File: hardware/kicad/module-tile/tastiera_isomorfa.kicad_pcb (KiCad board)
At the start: 2 copper layers, 87 x 97.2 mm, 67 parts, among them J101 Conn_LEFT, J102 Conn_TOP, J103 Conn_BOTTOM, J104 Conn_RIGHT, J105 BTNs_L_MSB, J106 BTNs_L_LSB, J107 BTNs_MSB, J108 BTNs_LSB, SW101 SW_Push, SW102 SW_Push, SW103 SW_Push, SW104 SW_Push, SW105 SW_Push, SW106 SW_Push, SW107 SW_Push, SW108 SW_Push, SW109 SW_Push, SW110 SW_Push, SW111 SW_Push, SW112 SW_Push, U101 74AUC2G126, U102 74AUC2G08, U103 74HC165, U104 74HC165, U105 74AHC1G04, U106 74LVC2G32, U107 74AUC2G125, U108 74LVC2G74, U109 74LS161

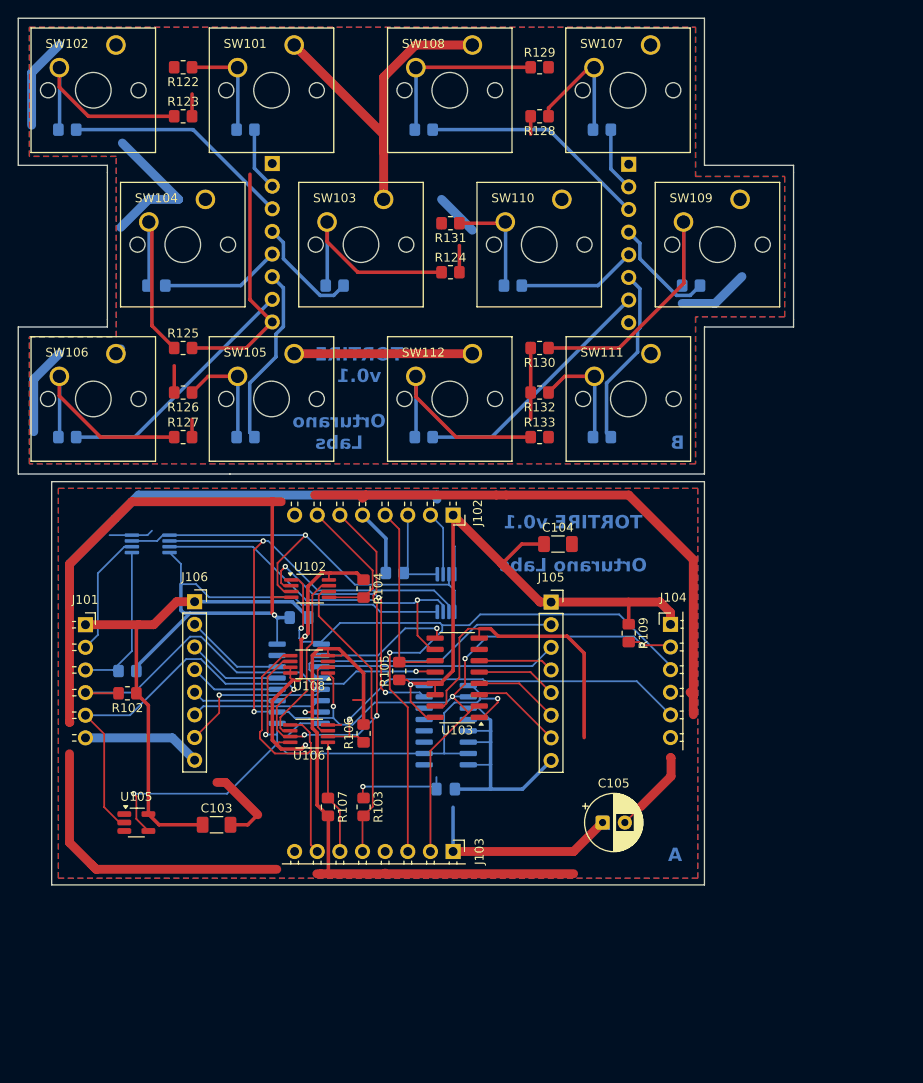
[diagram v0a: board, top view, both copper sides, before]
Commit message: Create gerber files
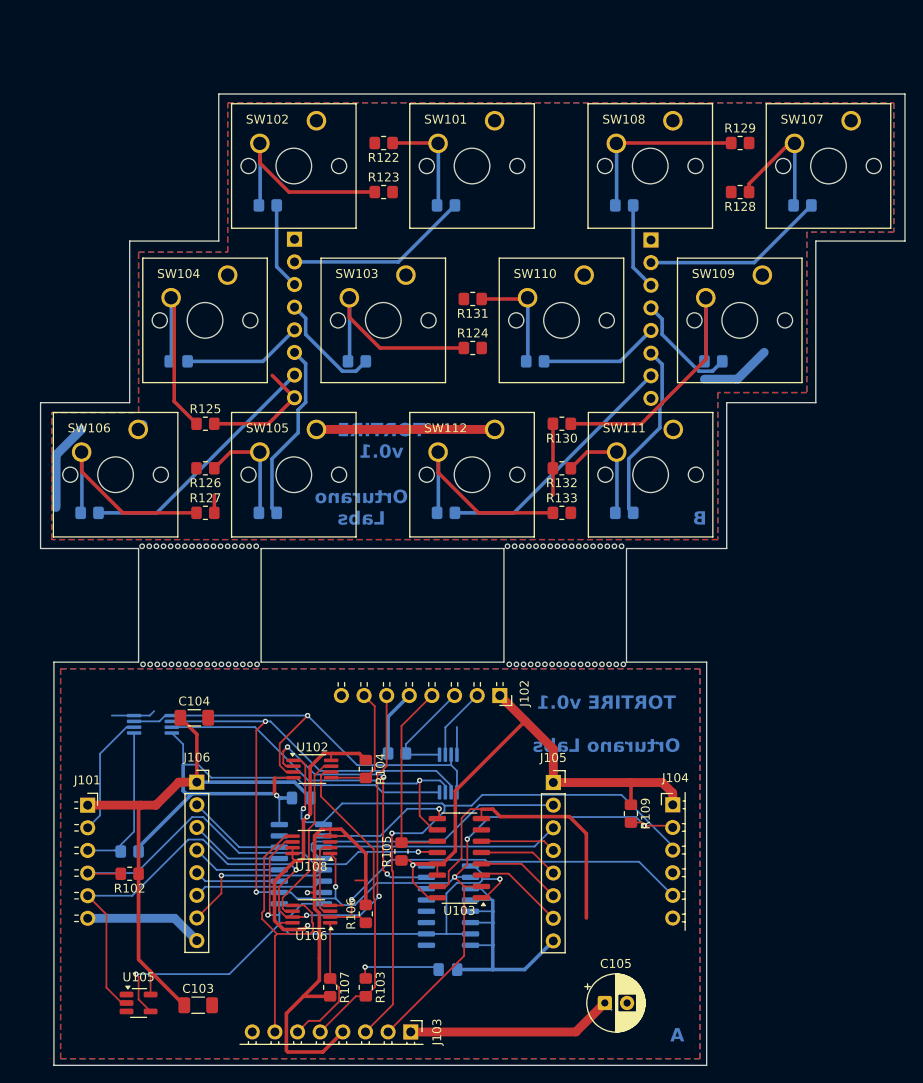
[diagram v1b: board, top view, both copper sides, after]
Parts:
- added REF**10: Senza-titolo, Senza-titolo, F.Cu at (124.5, 95.8)
- added REF**10: Senza-titolo, Senza-titolo, F.Cu at (166.5, 109.0)
- added REF**10: Senza-titolo, Senza-titolo, F.Cu at (124.6, 109.0)
- added REF**10: Senza-titolo, Senza-titolo, F.Cu at (165.5, 95.8)
- added REF**11: Senza-titolo, Senza-titolo, F.Cu at (125.3, 95.8)
- added REF**11: Senza-titolo, Senza-titolo, F.Cu at (166.3, 95.8)
- added REF**11: Senza-titolo, Senza-titolo, F.Cu at (167.3, 109.0)
- added REF**11: Senza-titolo, Senza-titolo, F.Cu at (125.4, 109.0)
- added REF**12: Senza-titolo, Senza-titolo, F.Cu at (126.1, 95.8)
- added REF**12: Senza-titolo, Senza-titolo, F.Cu at (126.2, 109.0)
- added REF**12: Senza-titolo, Senza-titolo, F.Cu at (168.1, 109.0)
- added REF**12: Senza-titolo, Senza-titolo, F.Cu at (167.1, 95.8)
- added REF**13: Senza-titolo, Senza-titolo, F.Cu at (167.9, 95.8)
- added REF**13: Senza-titolo, Senza-titolo, F.Cu at (168.9, 109.0)
- added REF**13: Senza-titolo, Senza-titolo, F.Cu at (127.0, 109.0)
- added REF**13: Senza-titolo, Senza-titolo, F.Cu at (126.9, 95.8)
- added REF**14: Senza-titolo, Senza-titolo, F.Cu at (127.7, 95.8)
- added REF**14: Senza-titolo, Senza-titolo, F.Cu at (169.7, 109.0)
- added REF**14: Senza-titolo, Senza-titolo, F.Cu at (127.8, 109.0)
- added REF**14: Senza-titolo, Senza-titolo, F.Cu at (168.7, 95.8)
- added REF**15: Senza-titolo, Senza-titolo, F.Cu at (169.5, 95.8)
- added REF**15: Senza-titolo, Senza-titolo, F.Cu at (128.5, 95.8)
- added REF**15: Senza-titolo, Senza-titolo, F.Cu at (170.5, 109.0)
- added REF**15: Senza-titolo, Senza-titolo, F.Cu at (128.6, 109.0)
- added REF**16: Senza-titolo, Senza-titolo, F.Cu at (170.3, 95.8)
- added REF**16: Senza-titolo, Senza-titolo, F.Cu at (129.3, 95.8)
- added REF**16: Senza-titolo, Senza-titolo, F.Cu at (171.3, 109.0)
- added REF**16: Senza-titolo, Senza-titolo, F.Cu at (129.4, 109.0)
- added REF**17: Senza-titolo, Senza-titolo, F.Cu at (172.1, 109.0)
- added REF**17: Senza-titolo, Senza-titolo, F.Cu at (171.1, 95.8)
- added REF**17: Senza-titolo, Senza-titolo, F.Cu at (130.2, 109.0)
- added REF**17: Senza-titolo, Senza-titolo, F.Cu at (130.1, 95.8)
- added REF**18: Senza-titolo, Senza-titolo, F.Cu at (172.9, 109.0)
- added REF**18: Senza-titolo, Senza-titolo, F.Cu at (131.0, 109.0)
- added REF**18: Senza-titolo, Senza-titolo, F.Cu at (171.9, 95.8)
- added REF**18: Senza-titolo, Senza-titolo, F.Cu at (130.9, 95.8)
- added REF**19: Senza-titolo, Senza-titolo, F.Cu at (131.8, 109.0)
- added REF**19: Senza-titolo, Senza-titolo, F.Cu at (172.7, 95.8)
- added REF**19: Senza-titolo, Senza-titolo, F.Cu at (131.7, 95.8)
- added REF**2: Senza-titolo, Senza-titolo, F.Cu at (160.1, 109.0)
- added REF**3: Senza-titolo, Senza-titolo, F.Cu at (159.9, 95.8)
- added REF**3: Senza-titolo, Senza-titolo, F.Cu at (118.9, 95.8)
- added REF**3: Senza-titolo, Senza-titolo, F.Cu at (119.0, 109.0)
- added REF**3: Senza-titolo, Senza-titolo, F.Cu at (160.9, 109.0)
- added REF**4: Senza-titolo, Senza-titolo, F.Cu at (119.7, 95.8)
- added REF**4: Senza-titolo, Senza-titolo, F.Cu at (119.8, 109.0)
- added REF**4: Senza-titolo, Senza-titolo, F.Cu at (160.7, 95.8)
- added REF**4: Senza-titolo, Senza-titolo, F.Cu at (161.7, 109.0)
- added REF**5: Senza-titolo, Senza-titolo, F.Cu at (162.5, 109.0)
- added REF**5: Senza-titolo, Senza-titolo, F.Cu at (120.6, 109.0)
- added REF**5: Senza-titolo, Senza-titolo, F.Cu at (120.5, 95.8)
- added REF**5: Senza-titolo, Senza-titolo, F.Cu at (161.5, 95.8)
- added REF**6: Senza-titolo, Senza-titolo, F.Cu at (121.3, 95.8)
- added REF**6: Senza-titolo, Senza-titolo, F.Cu at (121.4, 109.0)
- added REF**6: Senza-titolo, Senza-titolo, F.Cu at (162.3, 95.8)
- added REF**6: Senza-titolo, Senza-titolo, F.Cu at (163.3, 109.0)
- added REF**7: Senza-titolo, Senza-titolo, F.Cu at (122.1, 95.8)
- added REF**7: Senza-titolo, Senza-titolo, F.Cu at (122.2, 109.0)
- added REF**7: Senza-titolo, Senza-titolo, F.Cu at (164.1, 109.0)
- added REF**7: Senza-titolo, Senza-titolo, F.Cu at (163.1, 95.8)
- added REF**8: Senza-titolo, Senza-titolo, F.Cu at (163.9, 95.8)
- added REF**8: Senza-titolo, Senza-titolo, F.Cu at (123.0, 109.0)
- added REF**8: Senza-titolo, Senza-titolo, F.Cu at (164.9, 109.0)
- added REF**8: Senza-titolo, Senza-titolo, F.Cu at (122.9, 95.8)
- added REF**9: Senza-titolo, Senza-titolo, F.Cu at (123.7, 95.8)
- added REF**9: Senza-titolo, Senza-titolo, F.Cu at (164.7, 95.8)
- added REF**9: Senza-titolo, Senza-titolo, F.Cu at (165.7, 109.0)
- added REF**9: Senza-titolo, Senza-titolo, F.Cu at (123.8, 109.0)
- moved C104 45.2 mm to (124.8, 115.0)
- moved SW102 24.1 mm to (138.5, 48.0)
- moved R110 24.1 mm to (153.0, 57.5)
- moved R111 24.1 mm to (133.0, 57.5)
- moved R116 24.1 mm to (193.0, 57.5)
- moved R117 24.1 mm to (173.0, 57.5)
- moved R122 24.1 mm to (146.0, 50.5)
- moved R123 24.1 mm to (146.0, 56.0)
- moved R128 24.1 mm to (186.0, 56.0)
- moved R129 24.1 mm to (186.0, 50.5)
- moved SW101 24.1 mm to (158.5, 48.0)
- moved SW107 24.1 mm to (198.5, 48.0)
- moved SW108 24.1 mm to (178.5, 48.0)
- moved J102 20.9 mm to (159.0, 112.5)
- moved J103 20.8 mm to (149.0, 150.2)
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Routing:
- net GND: track 406.1 -> 215.2 mm
- net VCC_T: track 113.7 -> 39.3 mm
- net VCC: track 261.8 -> 209.1 mm
- net GND_T: track 49.3 -> 24.7 mm
- net /keyboard/BTNs1: track 25.7 -> 9.71 mm
- net /keyboard/BTNs7: track 25.7 -> 9.79 mm
- net /keyboard/BTNs0: track 7.17 -> 20.6 mm
- net /keyboard/BTNs6: track 7.25 -> 20.7 mm
- net /tile/T_data: track 10.5 -> 13.5 mm
- net /tile/B_first: track 33.1 -> 36.0 mm
- net /tile/B_latch: track 12.8 -> 15.3 mm
- net Net-(U109-Tc): track 33.1 -> 35.4 mm
- net /tile/T_W: track 16.1 -> 14.1 mm
- net /tile/B_clk: track 138.8 -> 140.7 mm
- net /tile/L_latch: track 83.9 -> 82.4 mm
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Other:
- board size 87 x 97.2 mm -> 97 x 109 mm
